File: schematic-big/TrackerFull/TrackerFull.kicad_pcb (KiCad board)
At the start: 2 copper layers, 43.2 x 38.1 mm, 58 parts, among them J1 Conn_01x05_Male, J3 Screw_Terminal_01x02, J4 78646-3001, J5 Screw_Terminal_01x02, Q1 IRLML0030, Q2 IRLML5203, Q3 IRLML5203, SW1 SW_Push, U1 LP2985-3.3, U2 LIS3DSH, U3 ATtiny85-20PU, U4 MCP73831-2-OT, U5 U.FL

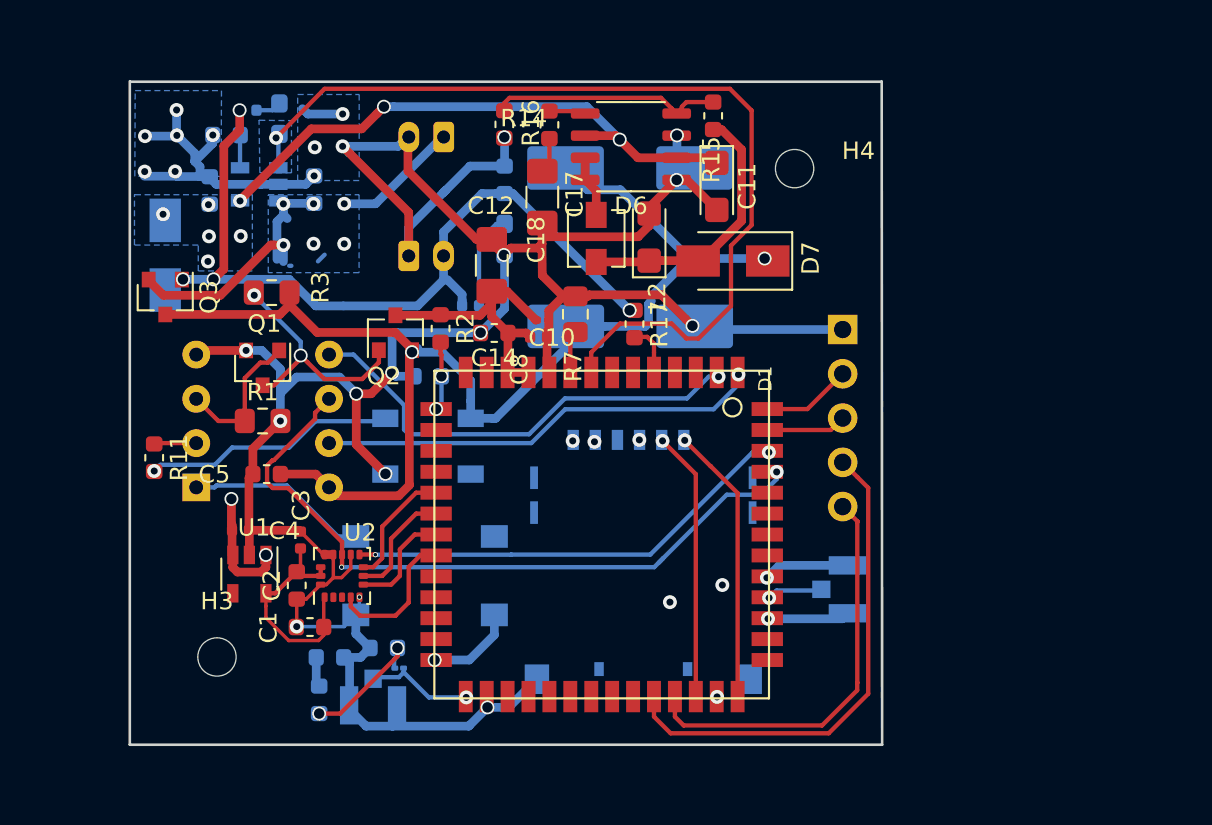
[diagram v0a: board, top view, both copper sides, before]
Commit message: last changes
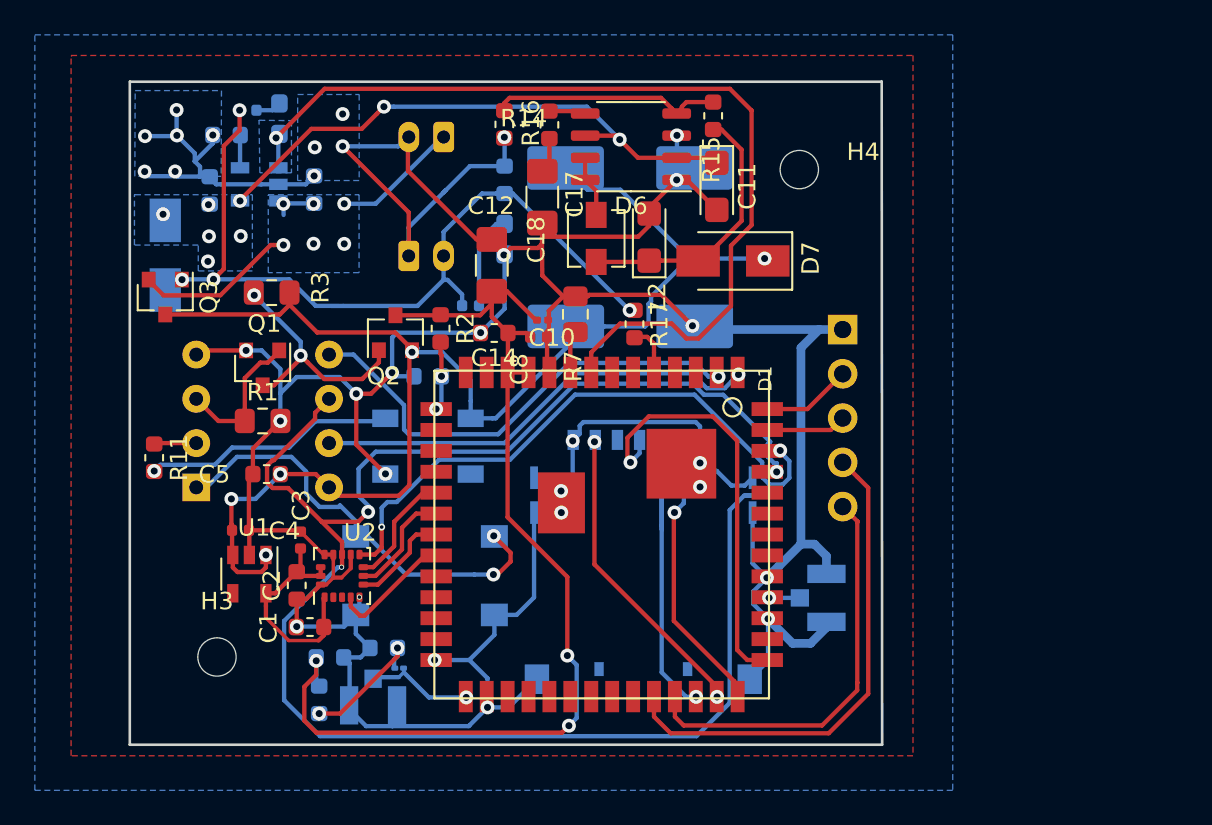
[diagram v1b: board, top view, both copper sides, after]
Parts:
- moved GSM1 1.33 mm to (203.9, 96.0)
- moved H4 0.28 mm to (202.3, 71.5)
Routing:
- net GNDREF: track 195.4 -> 256.1 mm, vias 28 -> 32
- net /ACCEL_INT1: track 41.3 -> 98.0 mm, vias 2 -> 3
- net /VBAT: track 19.1 -> 60.5 mm, vias 0 -> 3
- net /SIM_RST: track 0.00 -> 24.3 mm
- net /VSIM: track 0.00 -> 17.6 mm
- net /AVR_RST: track 10.4 -> 25.1 mm, vias 0 -> 2
- net /ACCEL_INT2: track 25.9 -> 34.4 mm
- net /SIM_IO: track 15.5 -> 21.1 mm
- net /V_BAT: track 23.9 -> 19.3 mm
- net BAT_IN: track 77.6 -> 81.0 mm, vias 4 -> 5
- net Net-(D1-Pad45): track 3.20 -> 1.76 mm
- net +5V: track 47.0 -> 48.2 mm
- net /ACCEL_SCL: track 8.27 -> 7.08 mm
- net /AVR_MOSI_SDA: track 26.4 -> 27.1 mm
- net /SIM_CLK: track 16.0 -> 16.6 mm
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- added copper zone on B.Cu, net BAT_IN
- added copper zone on F.Cu, net GNDREF
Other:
- outline, holes or cut-outs redrawn
- net class Default: clearance 0.2 -> 0.127
- rule trace_clearance: 0.2 -> 0.127
- rule trace_min: 0.2 -> 0.127
- rule via_min_drill: 0.3 -> 0.2
- rule via_min_size: 0.4 -> 0.2

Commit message: last changes
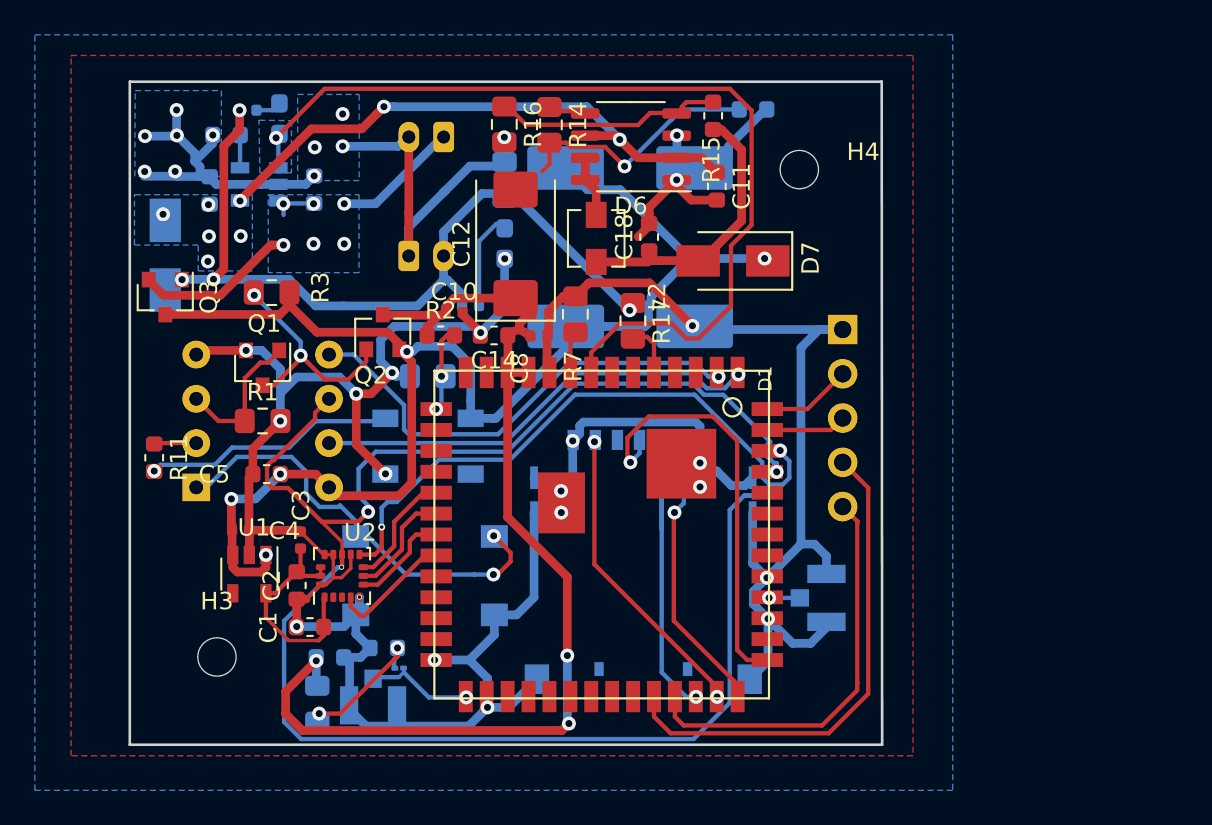
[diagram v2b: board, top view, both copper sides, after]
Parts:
- C1: value 4.7u -> 4.7uF
- C10: footprint Capacitor_SMD:C_0201_0603Metric -> Capacitor_SMD:C_0402_1005Metric
- C11, C18: footprint Capacitor_Tantalum_SMD:CP_EIA-3216-18_Kemet-A -> Capacitor_SMD:C_0603_1608Metric
- C12: footprint Capacitor_SMD:C_1206_3216Metric_Pad1.42x1.75mm_HandSolder -> Capacitor_Tantalum_SMD:CP_EIA-7343-31_Kemet-D
- C17: footprint Capacitor_SMD:C_1206_3216Metric_Pad1.42x1.75mm_HandSolder -> Capacitor_SMD:C_0603_1608Metric; moved to B.Cu
- C6: value C -> 4.7uF
- R10: value 100kOm -> 100K; footprint Resistor_SMD:R_0603_1608Metric -> Resistor_SMD:R_0805_2012Metric_Pad1.15x1.40mm_HandSolder
- R13, R17, R4: footprint Resistor_SMD:R_0603_1608Metric -> Resistor_SMD:R_0805_2012Metric_Pad1.15x1.40mm_HandSolder
- R14, R16: value 10000 -> 10K; footprint Resistor_SMD:R_0603_1608Metric -> Resistor_SMD:R_0805_2012Metric_Pad1.15x1.40mm_HandSolder
- R15: value 43000 -> 43K
- moved C17 13.1 mm to (199.6, 68.0), turned to 180 degrees
- moved C10 5.09 mm to (182.5, 79.6)
- moved C12 1.84 mm to (186.0, 75.7)
- moved Q2 0.73 mm to (178.4, 80.8)
- moved R2 0.40 mm to (181.7, 81.0), turned to 0 degrees
- moved D2 0.26 mm to (185.4, 75.7)
- moved R13 0.25 mm to (174.6, 102.1)
- moved R17 0.20 mm to (192.8, 80.1)
- moved C14 0.14 mm to (184.8, 81.0)
- moved C8 0.06 mm to (187.4, 81.0)
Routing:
- net GNDREF: track 256.1 -> 241.7 mm
- net Net-(C17-Pad2): track 2.04 -> 14.9 mm, vias 0 -> 1
- net Net-(D1-Pad15): track 4.34 -> 5.27 mm
- net /ACCEL_INT1: track 98.0 -> 98.9 mm
- net /VBAT: track 60.5 -> 59.7 mm
- net Net-(Q1-Pad3): track 13.7 -> 13.0 mm
- net BAT_IN: track 81.0 -> 81.6 mm

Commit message: schematic updated
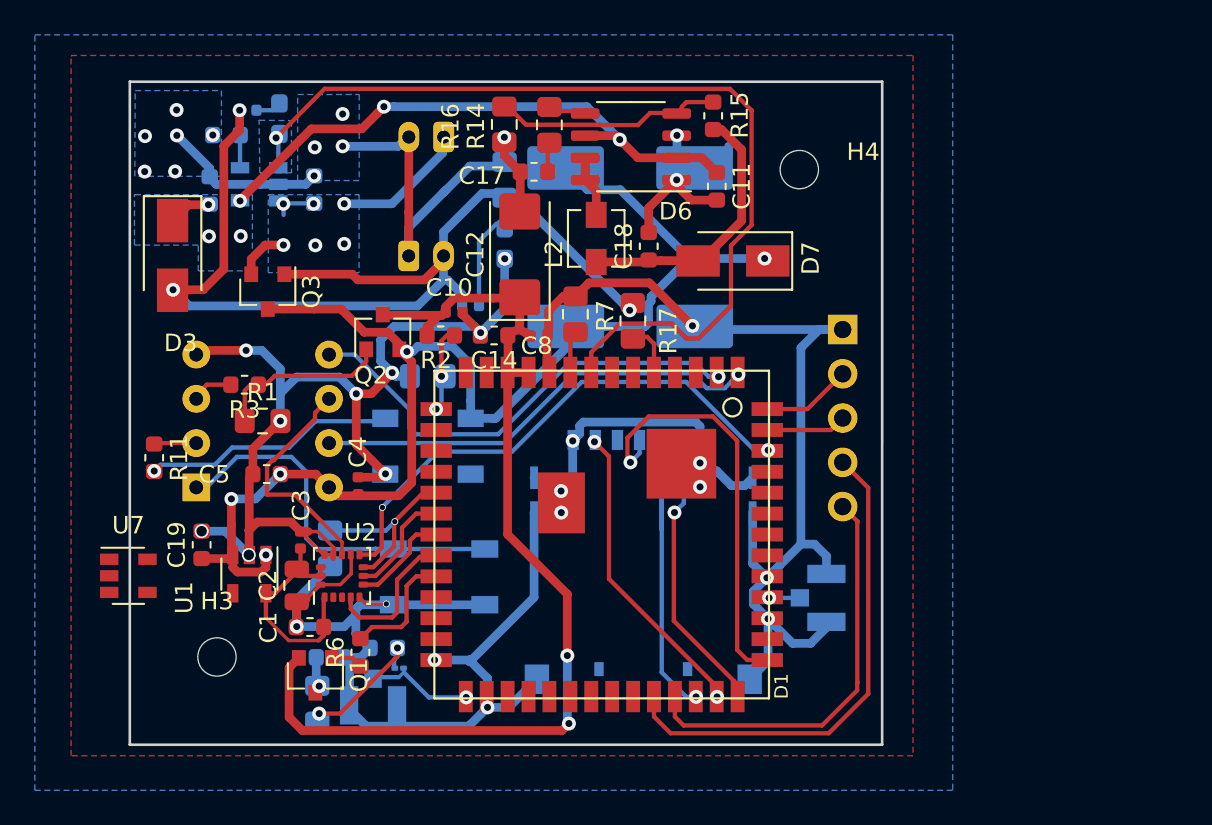
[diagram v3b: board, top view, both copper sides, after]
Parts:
- added C19: 1uF, Capacitor_SMD:C_0603_1608Metric, F.Cu at (168.0, 93.0)
- added R5: 10K, Resistor_SMD:R_0805_2012Metric_Pad1.15x1.40mm_HandSolder, B.Cu at (175.4, 93.2)
- added R6: 470, Resistor_SMD:R_0603_1608Metric, F.Cu at (177.1, 99.2)
- added U7: MIC5504-3.3YM5, Package_TO_SOT_SMD:SOT-23-5, F.Cu at (163.8, 94.8)
- C1: value 4.7uF -> 2.2uF
- C12: footprint Capacitor_Tantalum_SMD:CP_EIA-7343-31_Kemet-D -> Capacitor_Tantalum_SMD:CP_EIA-6032-28_Kemet-C
- C17, D3: moved to F.Cu
- C2: footprint Capacitor_SMD:C_0603_1608Metric -> Capacitor_SMD:C_0805_2012Metric
- Q1: value IRLML0030 -> DMG2305UXQ
- Q2, Q3: value IRLML5203 -> DMG2305UXQ
- R10: value 100K -> 10K
- R12, R8: value 250 -> 150
- R3: value 10K -> 470; footprint Resistor_SMD:R_0805_2012Metric_Pad1.15x1.40mm_HandSolder -> Resistor_SMD:R_0603_1608Metric
- SW1: value SW_Push -> PTS647SK38SMTR2LFS; footprint Button_Switch_SMD:SW_Push_1P1T_NO_6x6mm_H9.5mm -> imported:PTS647SK38SMTR2LFS
- U1: value LP2985-3.3 -> LP2980IM5-3.6
- moved Q1 17.9 mm to (174.5, 100.5)
- moved C17 13.1 mm to (187.1, 71.6), turned to 0 degrees
- moved C4 7.22 mm to (177.0, 89.6), turned to 270 degrees
- moved Q3 5.89 mm to (171.8, 78.5)
- moved R3 5.51 mm to (170.5, 83.8)
- moved SW1 0.81 mm to (181.6, 94.8)
- moved C12 0.65 mm to (186.3, 76.3)
- moved C18 0.52 mm to (193.7, 75.9)
- moved D3 0.42 mm to (166.3, 76.4)
- renumbered GSM1 to U6
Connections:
- net /3.3v renamed /3.6v
- C9 pad 1: /VBAT -> Net-(C9-Pad1)
- D1 pad 23: (no net) -> /GPS_POWER
- D1 pad 51: /ACCEL_INT1 -> (no net)
- Q1 pad 1: /PWR_CTRL -> Net-(Q1-Pad1)
- Q1 pad 2: GNDREF -> /VBAT
- Q1 pad 3: Net-(Q1-Pad3) -> Net-(C9-Pad1)
- Q2 pad 1: Net-(Q1-Pad3) -> /PWR_CTRL
- R13 pad 1: /VBAT -> Net-(C9-Pad1)
- R3 pad 1: BAT_IN -> /PWR_CTRL
- R3 pad 2: Net-(Q1-Pad3) -> Net-(R3-Pad2)
- SW1 pad 2: GNDREF -> /AVR_RST
- U3 pad 3: /PWR_CTRL -> Net-(R3-Pad2)
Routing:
- net /ACCEL_INT1: track 98.9 -> 13.2 mm, vias 3 -> 0
- net Net-(C17-Pad2): track 14.9 -> 1.71 mm, vias 1 -> 0
- net Net-(Q1-Pad3): track 13.0 -> 0.00 mm, vias 2 -> 0
- net GNDREF: track 241.7 -> 253.7 mm, vias 32 -> 34
- net +5V: track 48.2 -> 58.6 mm, vias 4 -> 3
- net /GPS_POWER: track 0.00 -> 7.03 mm
- net /V_BAT: track 19.3 -> 13.6 mm
- net BAT_IN: track 81.6 -> 76.6 mm
- net /ACCEL_CS: track 6.77 -> 10.7 mm, vias 0 -> 1
- net /ACCEL_INT2: track 34.4 -> 30.5 mm
- net /AVR_RST: track 25.1 -> 21.8 mm, vias 2 -> 0
- net Net-(R3-Pad2): track 0.00 -> 2.60 mm
- net /CHARGER_VDD: track 33.3 -> 35.7 mm, vias 8 -> 6
- net /PWR_CTRL: track 8.43 -> 10.8 mm
- net Net-(C9-Pad1): track 0.00 -> 2.19 mm, vias 0 -> 1
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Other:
- board size 43.2 x 38.1 mm -> 43.2 x 38 mm
- rule via_min_drill: 0.2 -> 0.3
- rule via_min_size: 0.2 -> 0.3

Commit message: next milestone
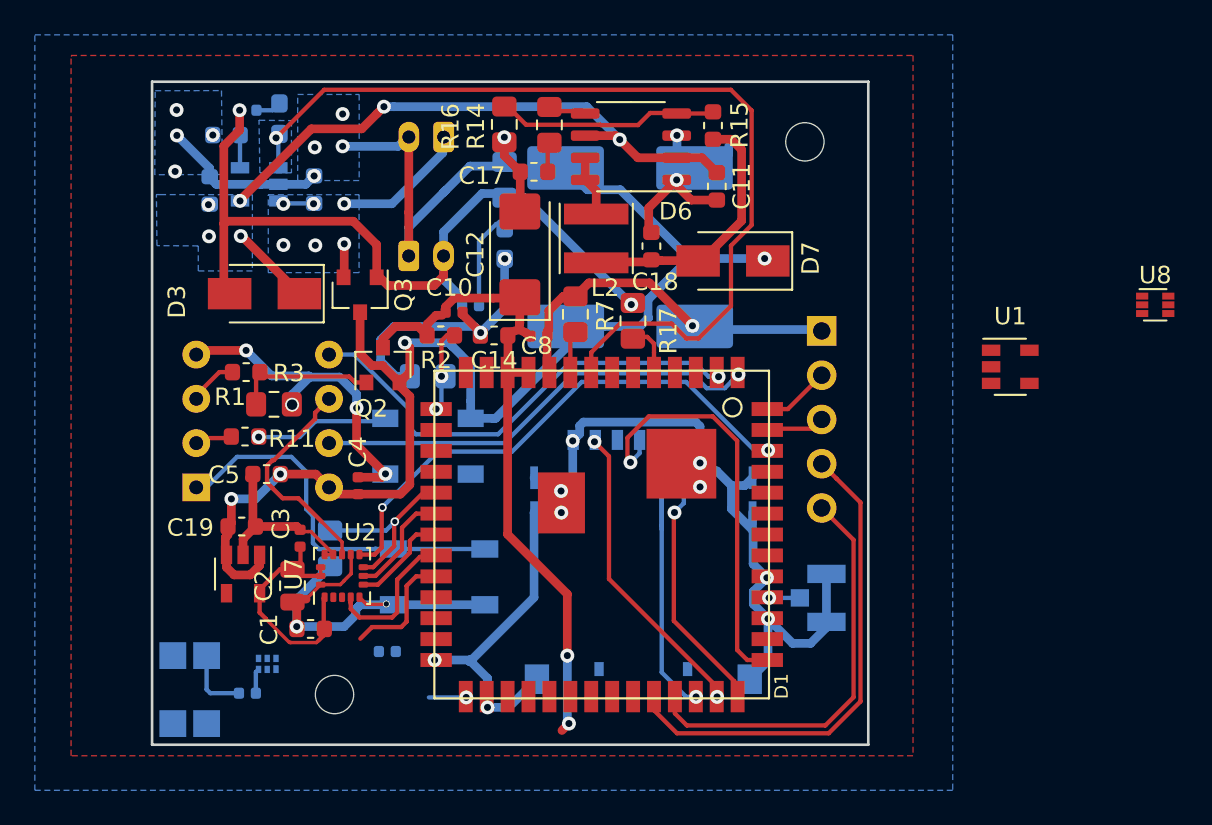
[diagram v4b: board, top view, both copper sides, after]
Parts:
- removed C13, C9: 4.7uF, Capacitor_SMD:C_0603_1608Metric
- removed Q1: DMG2305UXQ, Package_TO_SOT_SMD:SOT-23
- removed R13: 100K, Resistor_SMD:R_0805_2012Metric_Pad1.15x1.40mm_HandSolder
- removed R6: 470, Resistor_SMD:R_0603_1608Metric
- added ANT1: 1462350001, imported:ANT_1462350001, B.Cu at (167.3, 101.3)
- added L3: LQG15HS1N8B02, Inductor_SMD:L_0402_1005Metric, B.Cu at (178.7, 99.1)
- added U8: AP62301, Package_TO_SOT_SMD:SOT-563, F.Cu at (222.7, 79.2)
- C1: value 2.2uF -> 0.47uF
- H3, H4: moved to B.Cu
- L1: value LQG15HN27NJ -> LQG15HS5N1B02; footprint Inductor_SMD:L_01005_0402Metric -> Inductor_SMD:L_0402_1005Metric
- L2: value IHLP1212BZER2R2M11 -> MDWK4040T3R3MM; footprint Inductor_SMD:L_Vishay_IHLP-1212 -> Inductor_SMD:L_Taiyo-Yuden_MD-4040
- U1: value LP2980IM5-3.6 -> TLV62568DBV
- U5: value U.FL -> BGU7007,115; footprint mailboxNotifier:U.FL -> imported:PSON50P100X145X50-6N
- U7: value MIC5504-3.3YM5 -> MIC5232-2.5YD5
- moved U1 45.3 mm to (214.4, 82.8), turned to 0 degrees
- moved L1 8.83 mm to (170.6, 101.5)
- moved H3 7.08 mm to (175.6, 101.6)
- moved U7 6.58 mm to (170.4, 94.7), turned to 270 degrees
- moved U5 6.52 mm to (171.8, 99.8)
- moved D3 5.71 mm to (171.6, 78.6), turned to 180 degrees
- moved R11 5.35 mm to (170.5, 86.8), turned to 0 degrees
- moved Q3 5.30 mm to (177.1, 78.6)
- moved C19 2.53 mm to (170.3, 91.9), turned to 0 degrees
- moved Q2 1.90 mm to (178.4, 82.7)
- moved H4 1.62 mm to (202.6, 69.9)
- moved J1 1.21 mm to (203.6, 80.7)
- moved R1 1.16 mm to (172.2, 84.9)
- moved R3 0.73 mm to (170.6, 83.1)
- moved R15 0.56 mm to (197.4, 68.9)
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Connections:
- C1 pad 1: /3.6v -> /2.5v
- C2 pad 2: /3.6v -> /2.5v
- C3 pad 2: /3.6v -> /2.5v
- L1 pad 2: /GPS_RF -> Net-(L1-Pad2)
- U1 pad 1: BAT_IN -> (no net)
- U1 pad 2: GNDREF -> (no net)
- U1 pad 3: BAT_IN -> (no net)
- U1 pad 5: /3.6v -> (no net)
- U2 pad 1: /3.6v -> /2.5v
- U2 pad 14: /3.6v -> /2.5v
- U2 pad 15: /3.6v -> /2.5v
- U5 pad 3: /GPS_RF -> Net-(L1-Pad2)
- U7 pad 1: (no net) -> BAT_IN
- U7 pad 2: (no net) -> GNDREF
- U7 pad 3: (no net) -> BAT_IN
- U7 pad 5: (no net) -> /2.5v
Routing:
- net GNDREF: track 253.7 -> 207.8 mm, vias 34 -> 29
- net /VBAT: track 58.2 -> 38.7 mm
- net /2.5v: track 0.00 -> 13.1 mm
- net /3.6v: track 13.1 -> 0.00 mm
- net +5V: track 58.6 -> 47.1 mm, vias 3 -> 2
- net /LED_CTL: track 14.5 -> 7.71 mm
- net BAT_IN: track 76.6 -> 71.9 mm, vias 5 -> 4
- net /GPS_RF: track 6.27 -> 2.14 mm
- net Net-(ANT1-Pad1): track 7.57 -> 3.89 mm, vias 2 -> 0
- net /PWR_CTRL: track 10.8 -> 8.30 mm
- net /CHARGER_VDD: track 35.7 -> 38.0 mm
- net Net-(C9-Pad1): track 2.19 -> 0.00 mm, vias 1 -> 0
- net Net-(Q1-Pad1): track 1.83 -> 0.00 mm
- net /V_BAT: track 13.6 -> 11.8 mm
- net Net-(L1-Pad2): track 0.00 -> 1.43 mm
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- added copper zone on F.Cu, net BAT_IN
- removed copper zone on B.Cu, net BAT_IN
- removed copper zone on F.Cu, net GNDREF
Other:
- board size 43.2 x 38 mm -> 41.1 x 38 mm
